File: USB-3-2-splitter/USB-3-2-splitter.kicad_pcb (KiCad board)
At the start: 4 copper layers, 41 x 29 mm, 35 parts, among them J1 USB_C_Receptacle_USB2.0_16P, J2 USB_C_Receptacle, J3 USB_C_Receptacle, Q1 IRLML6401, Q2 IRLML6401, Q3 IRLML6401, Q4 IRLML6401, U3 SRV05-4

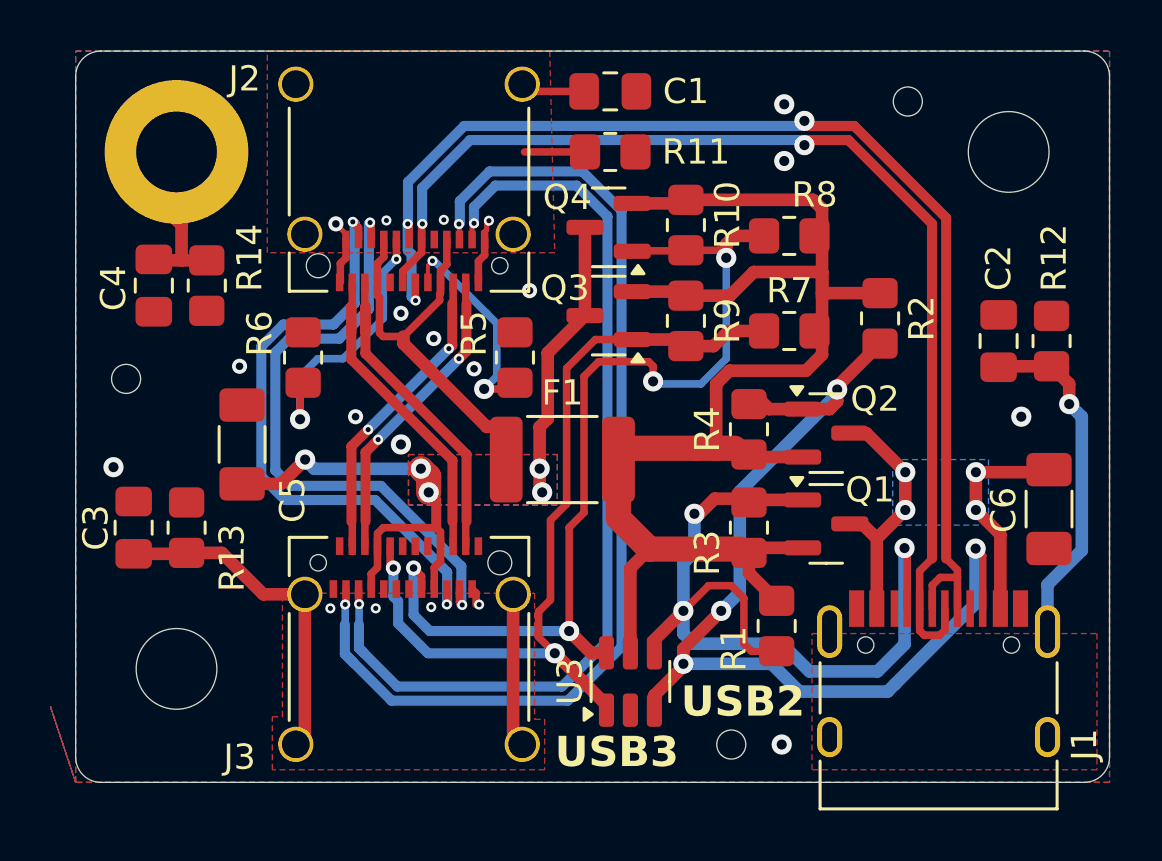
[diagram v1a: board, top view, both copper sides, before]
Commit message: More adjustments
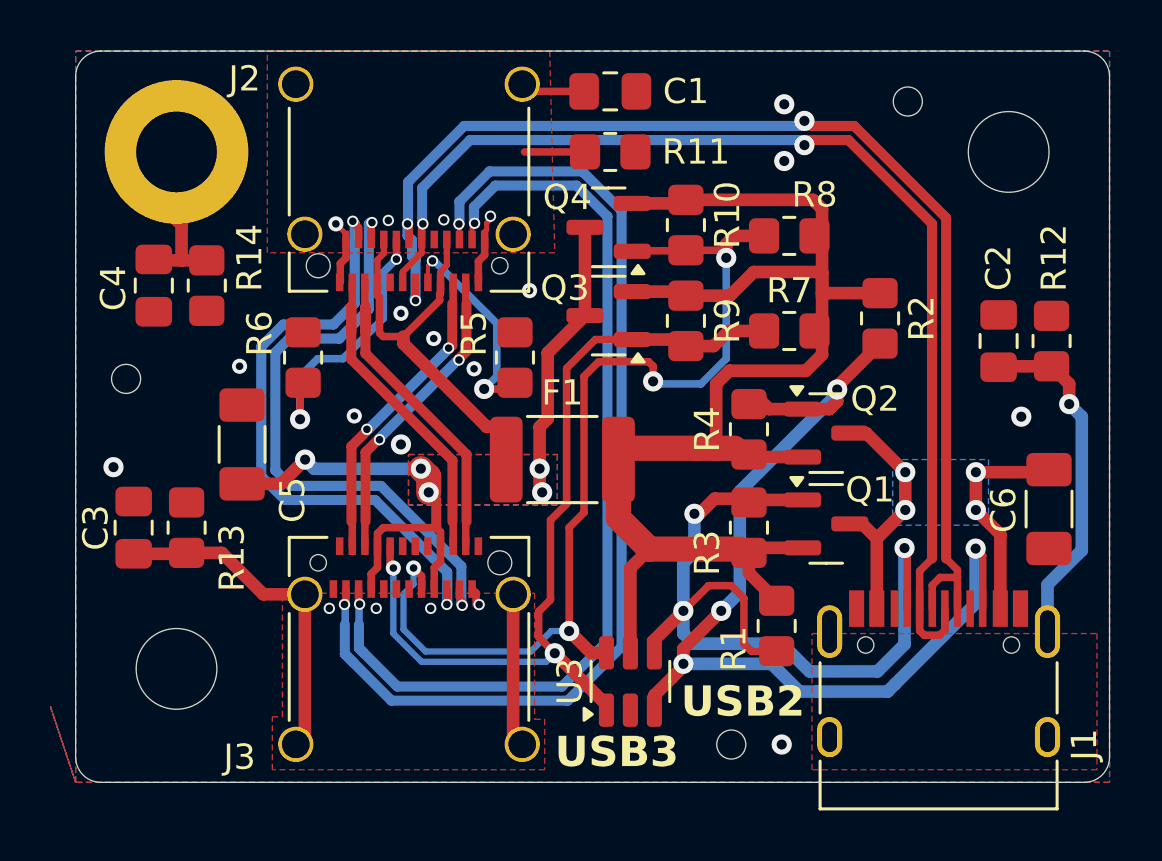
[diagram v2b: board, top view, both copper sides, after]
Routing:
- net CC2_USB3: track 37.8 -> 39.3 mm
- net CC1_USB3: track 33.7 -> 34.3 mm
